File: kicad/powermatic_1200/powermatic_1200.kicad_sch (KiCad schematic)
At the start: 61 parts, among them J1 T4171310004-001, J2 3PH-4W-PLUG, K1 HMC-9B30-11-DS, K2 HC3096N-52-900-24, K3 HMC-9B30-11-DS, K4 HMC-9B30-11-DS, K5 HMC-9B30-11-DS, K6 HMC-9B30-11-DS, M1 PWRM1200-MOTOR, Q1 FAZ-D4/2-NA-L, SW1 222102

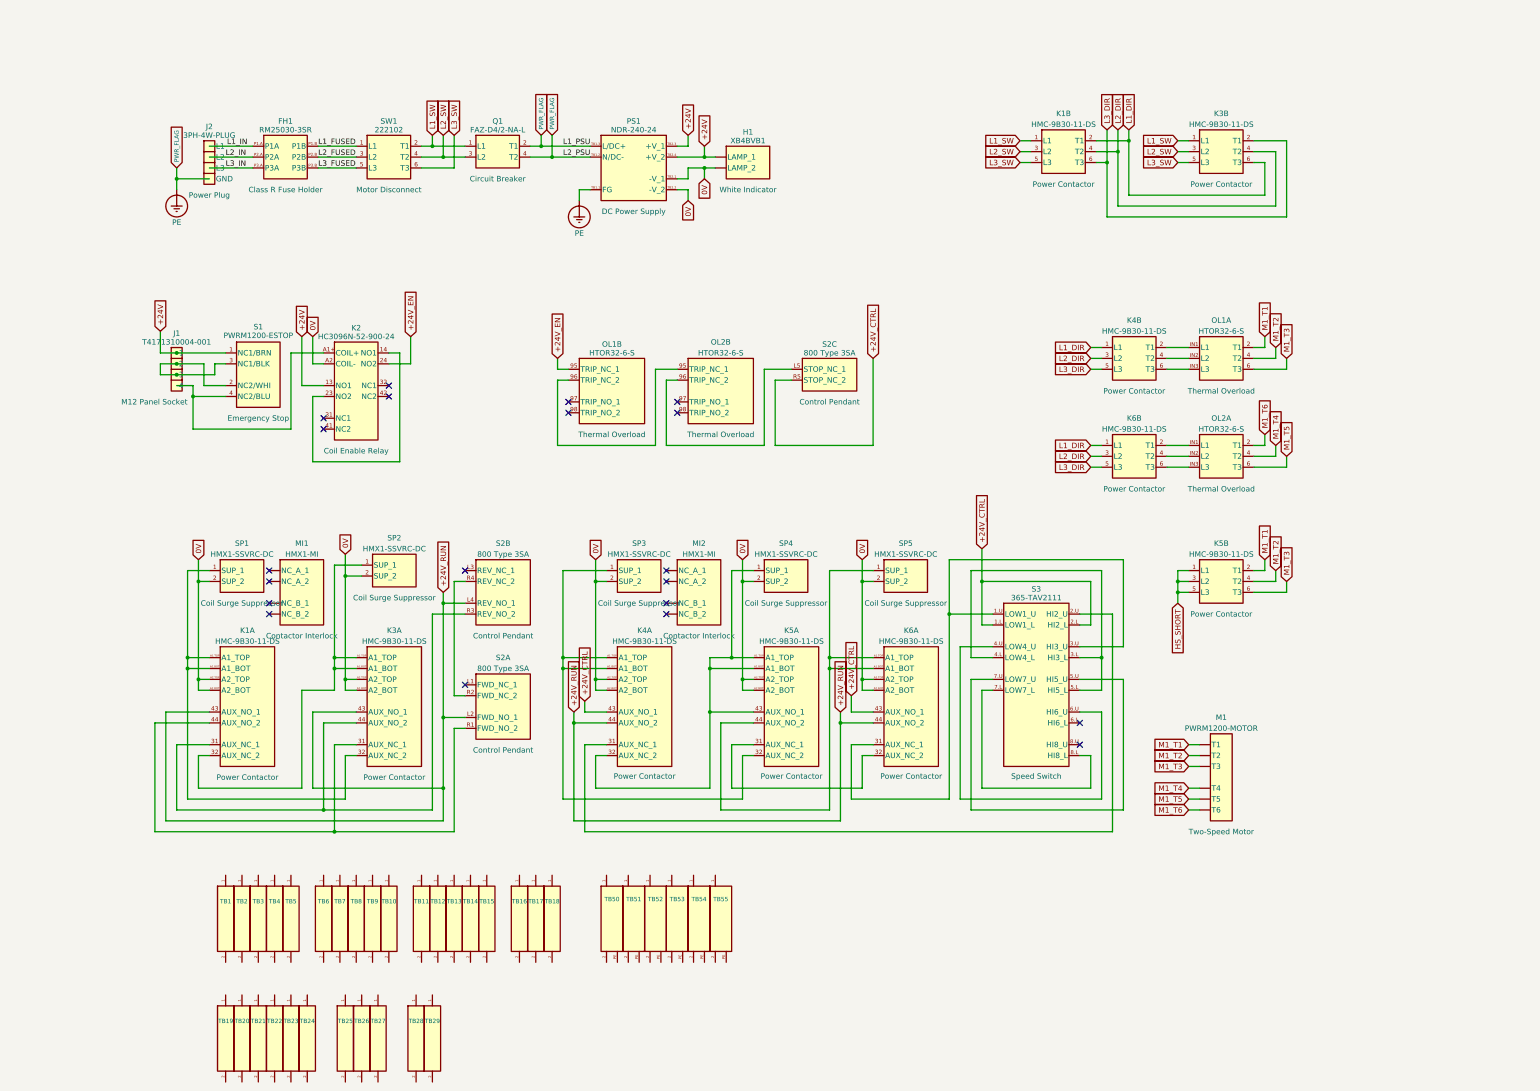
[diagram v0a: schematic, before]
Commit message: finalized panel layout
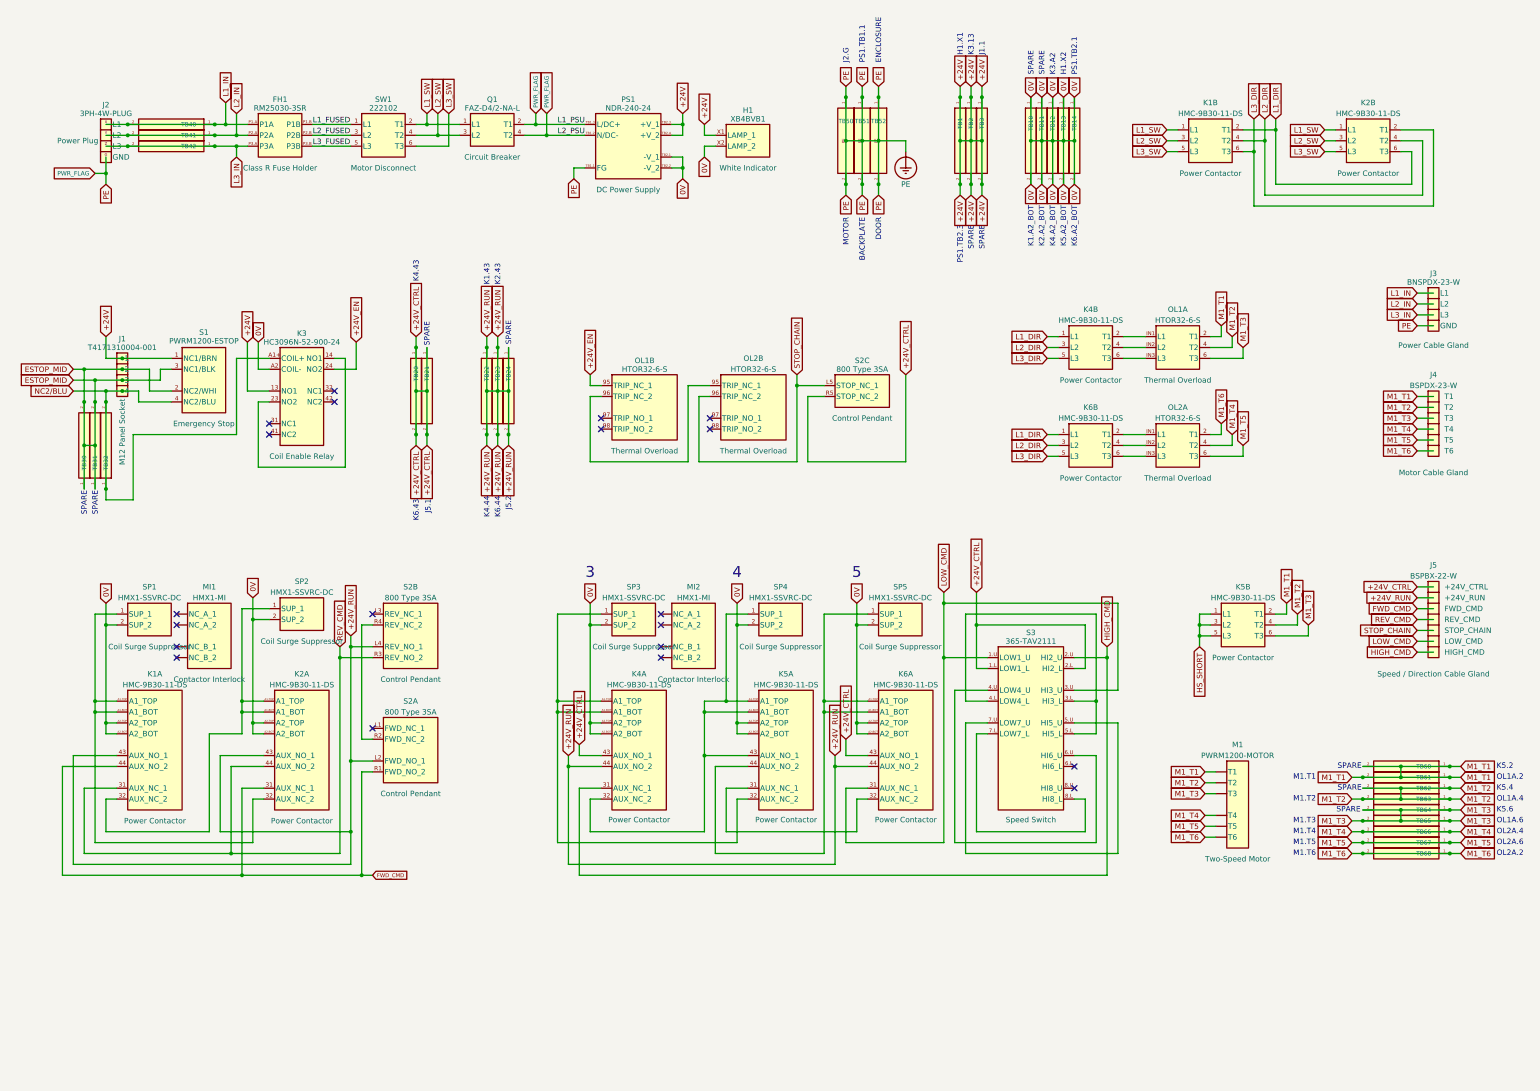
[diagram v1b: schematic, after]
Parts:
- removed TB10, TB11, TB17, TB19, TB8: KN-T12GRY-25, Controls:KN-T12GRY-25_Front, symbol Controls:KN-T12GRY-25
- removed TB50, TB51, TB52: KN-G12SP-10, Controls:KN-G12SP-10_Front, symbol Controls:KN-G12SP-10
- added J3: BNSPDX-23-W, Controls:BNSPDX-23-W_BottomWall, symbol Controls:BNSPDX-23-W
- added J4: BSPDX-23-W, Controls:BSPDX-23-W_BottomWall, symbol Controls:BSPDX-23-W
- added J5: BSPBX-22-W, Controls:BSPBX-22-W_BottomWall, symbol Controls:BSPBX-22-W
- added TB1, TB60, TB62, TB64: KN-T12GRY-25, Controls:KN-T12GRY-25_Front, symbol Controls:KN-T12GRY-25
- renumbered K3 to K2, K2 to K3, TB1 to TB10, TB3 to TB11, TB5 to TB12, TB7 to TB13, TB9 to TB14, TB13 to TB2, TB18 to TB20, TB20 to TB21, TB2 to TB22, TB4 to TB23, TB6 to TB24, TB15 to TB3, TB16 to TB30, TB14 to TB31, TB12 to TB32, TB23 to TB40, TB21 to TB41, TB22 to TB42, TB55 to TB50, TB54 to TB51, TB53 to TB52, TB24 to TB61, TB25 to TB63, TB26 to TB65, TB27 to TB66, TB28 to TB67, TB29 to TB68
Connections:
- net +24V: now also TB2.1 (TERM), TB2.2 (TERM), TB3.1 (TERM), TB3.2 (TERM), TB1.1 (TERM), TB1.2 (TERM)
- net +24V_CTRL: now also TB20.1 (TERM), TB20.2 (TERM), TB21.1 (TERM), TB21.2 (TERM), J5.1 (+24V_CTRL)
- net +24V_RUN: now also TB22.1 (TERM), TB22.2 (TERM), TB23.1 (TERM), TB23.2 (TERM), TB24.1 (TERM), TB24.2 (TERM), J5.2 (+24V_RUN)
- net 0V: now also TB10.1 (TERM), TB10.2 (TERM), TB11.1 (TERM), TB11.2 (TERM), TB12.1 (TERM), TB12.2 (TERM), TB13.1 (TERM), TB13.2 (TERM), TB14.1 (TERM), TB14.2 (TERM)
- net L1_IN: now also TB40.1 (TERM), TB40.2 (TERM), J3.X (L1)
- net L2_IN: now also TB41.1 (TERM), TB41.2 (TERM), J3.Y (L2)
- net L3_IN: now also TB42.1 (TERM), TB42.2 (TERM), J3.Z (L3)
- net M1_T1: now also TB61.1 (TERM), TB61.2 (TERM), J4.T1, TB60.1 (TERM), TB60.2 (TERM)
- net M1_T2: now also TB63.1 (TERM), TB63.2 (TERM), J4.T2, TB62.1 (TERM), TB62.2 (TERM)
- net M1_T3: now also TB65.1 (TERM), TB65.2 (TERM), J4.T3, TB64.1 (TERM), TB64.2 (TERM)
- net M1_T4: now also TB66.1 (TERM), TB66.2 (TERM), J4.T4
- net M1_T5: now also TB67.1 (TERM), TB67.2 (TERM), J4.T5
- net M1_T6: now also TB68.1 (TERM), TB68.2 (TERM), J4.T6
- net PE: now also TB50.1 (TERM), TB50.2 (TERM), TB50.PE, TB51.1 (TERM), TB51.2 (TERM), TB51.PE, TB52.1 (TERM), TB52.2 (TERM), TB52.PE, J3.G (GND)
- net NC2/BLU: now reaches TB32.1 (TERM)
- net NC2/BLU: now also J1.4, K3.A1+ (COIL+), S1.4 (NC2/BLU), TB32.2 (TERM)
- net LOW_CMD: now reaches K6.31 (AUX_NC_1), S3.1.U (LOW1_U), S3.3.U (HI3_U)
- net LOW_CMD: now also J5.6 (LOW_CMD)
- net FWD_CMD: now reaches K1.44 (AUX_NO_2), K2.31 (AUX_NC_1), S2.R1 (FWD_NO_2)
- net FWD_CMD: now also J5.3 (FWD_CMD)
- net REV_CMD: now reaches K1.31 (AUX_NC_1), K2.44 (AUX_NO_2), S2.R3 (REV_NO_2)
- net REV_CMD: now also J5.4 (REV_CMD)
- net ESTOP_MID: now reaches J1.2, J1.3, S1.2 (NC2/WHI), S1.3 (NC1/BLK)
- net ESTOP_MID: now also TB30.1 (TERM), TB30.2 (TERM), TB31.1 (TERM), TB31.2 (TERM)
- net STOP_CHAIN: now reaches OL2.96 (TRIP_NC_2), S2.L5 (STOP_NC_1)
- net STOP_CHAIN: now also J5.5 (STOP_CHAIN)
- net HIGH_CMD: now reaches K4.31 (AUX_NC_1), S3.2.U (HI2_U)
- net HIGH_CMD: now also J5.7 (HIGH_CMD)
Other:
- note added: "3"
- note added: "4"
- note added: "5"
- note added: "BACKPLATE"
- note added: "DOOR"
- note added: "ENCLOSURE"
- note added: "H1.X1"
- note added: "H1.X2"
- note added: "J1.1"
- note added: "J2.G"
- note added: "J5.1"
- note added: "J5.2"
- note added: "K1.43"
- note added: "K1.A2_BOT"
- note added: "K2.43"
- note added: "K2.A2_BOT"
- note added: "K3.13"
- note added: "K3.A2"
- note added: "K4.43"
- note added: "K4.44"
- note added: "K4.A2_BOT"
- note added: "K5.2"
- note added: "K5.4"
- note added: "K5.6"
- note added: "K5.A2_BOT"
- note added: "K6.43"
- note added: "K6.44"
- note added: "K6.A2_BOT"
- note added: "M1.T1"
- note added: "M1.T2"
- note added: "M1.T3"
- note added: "M1.T4"
- note added: "M1.T5"
- note added: "M1.T6"
- note added: "MOTOR"
- note added: "OL1A.2"
- note added: "OL1A.4"
- note added: "OL1A.6"
- note added: "OL2A.2"
- note added: "OL2A.4"
- note added: "OL2A.6"
- note added: "PS1.TB1.1"
- note added: "PS1.TB2.1"
- note added: "PS1.TB2.3"
- note added: "SPARE"
- moved on the sheet: FH1, J1, K1A, K1B, K2A, K2B, K3, K4A, K4B, K5A, K5B, K6A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
